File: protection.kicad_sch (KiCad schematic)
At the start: 29 parts, among them U21 LM339DR

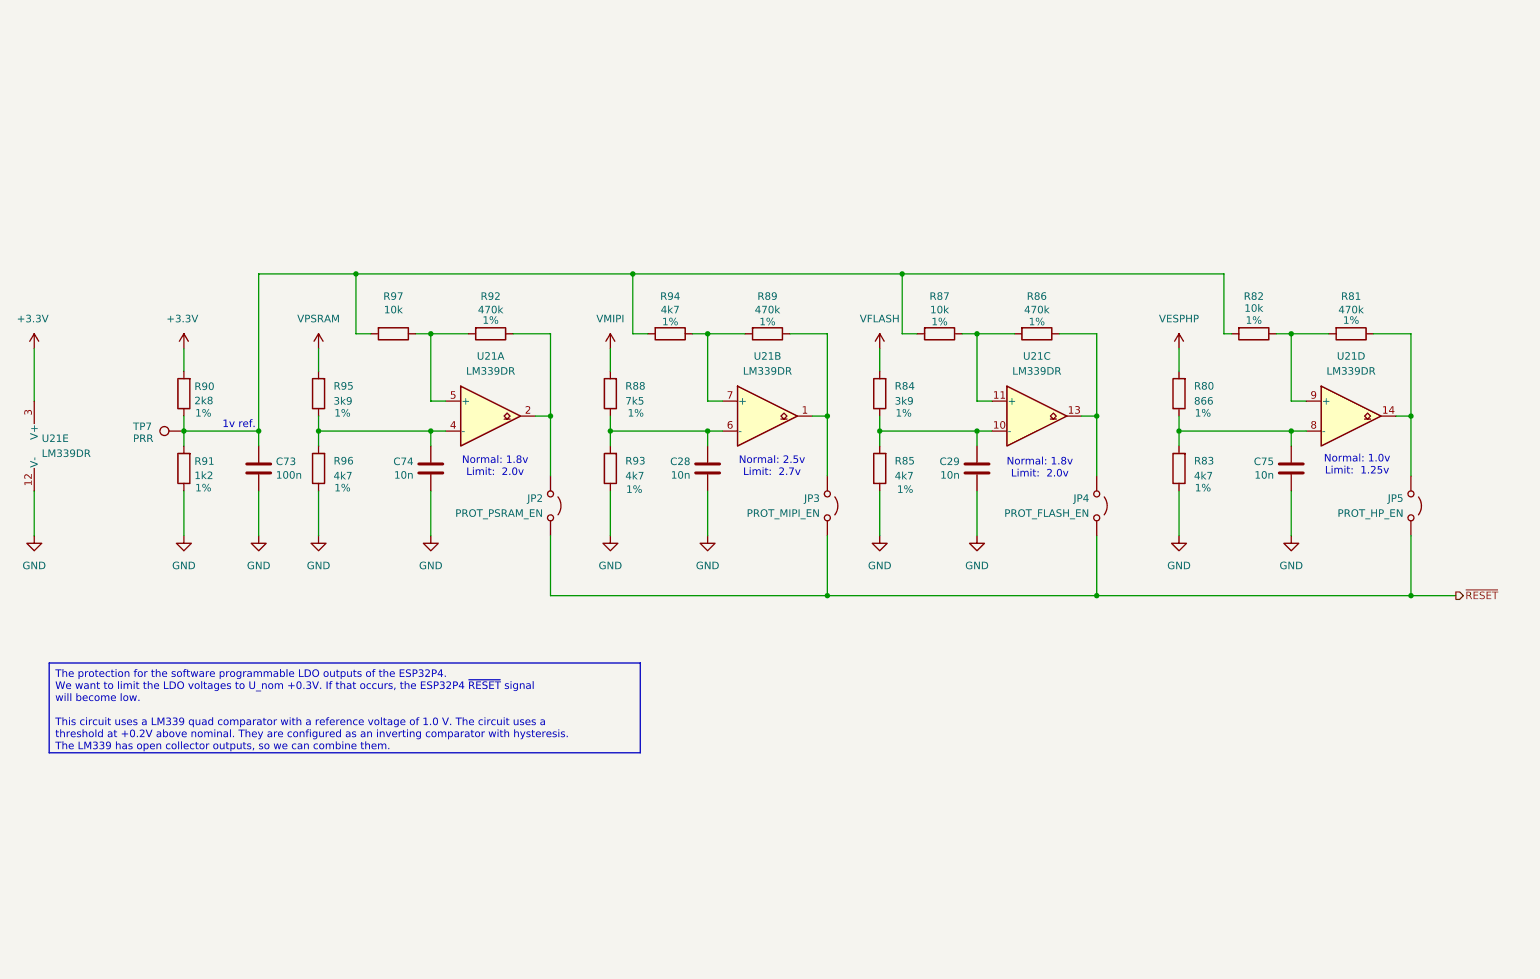
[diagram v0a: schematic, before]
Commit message: Replaced voltage comparitor circuit with zener setup. Also changed couple of 0.2mm vias to 0.3
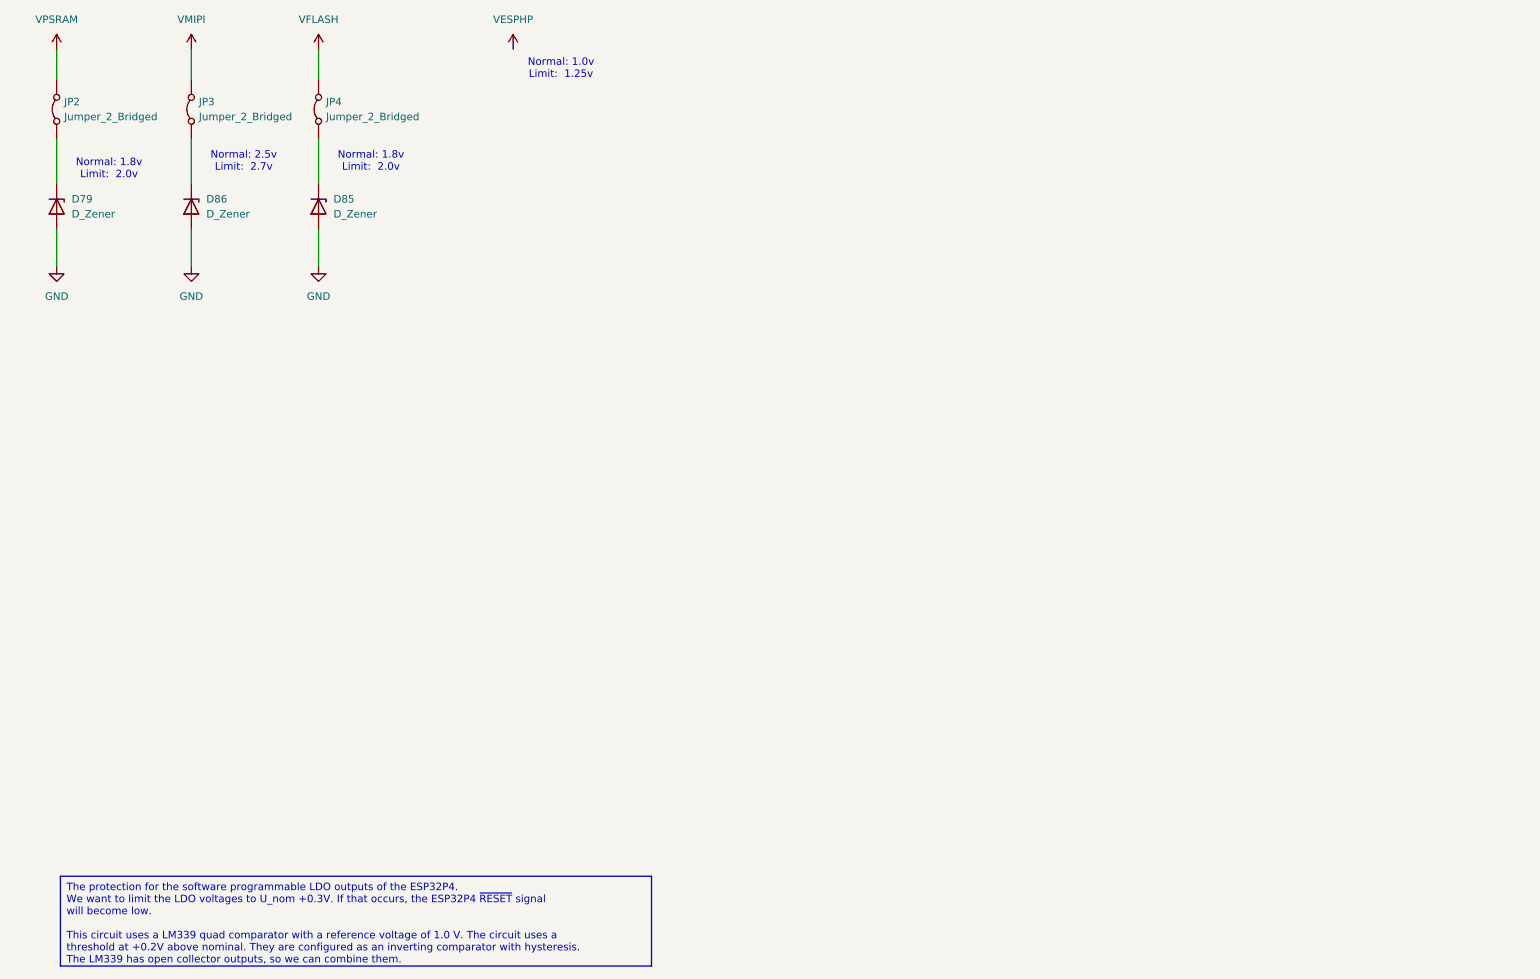
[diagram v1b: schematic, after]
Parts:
- removed C28, C29, C74, C75: 10n, Capacitor_SMD:C_0402_1005Metric, symbol symbols:C
- removed C73: 100n, Capacitor_SMD:C_0402_1005Metric, symbol symbols:C
- removed JP2: PROT_PSRAM_EN, Jumper:SolderJumper-2_P1.3mm_Open_RoundedPad1.0x1.5mm, symbol Jumper:Jumper_2_Open
- removed JP3: PROT_MIPI_EN, Jumper:SolderJumper-2_P1.3mm_Open_RoundedPad1.0x1.5mm, symbol Jumper:Jumper_2_Open
- removed JP4: PROT_FLASH_EN, Jumper:SolderJumper-2_P1.3mm_Open_RoundedPad1.0x1.5mm, symbol Jumper:Jumper_2_Open
- removed JP5: PROT_HP_EN, Jumper:SolderJumper-2_P1.3mm_Open_RoundedPad1.0x1.5mm, symbol Jumper:Jumper_2_Open
- removed R80: 866, Resistor_SMD:R_0402_1005Metric, symbol Device:R
- removed R81, R86, R89, R92: 470k, Resistor_SMD:R_0402_1005Metric, symbol Device:R
- removed R82, R87, R97: 10k, Resistor_SMD:R_0402_1005Metric, symbol Device:R
- removed R83, R85, R93, R94, R96: 4k7, Resistor_SMD:R_0402_1005Metric, symbol Device:R
- removed R84, R95: 3k9, Resistor_SMD:R_0402_1005Metric, symbol Device:R
- removed R88: 7k5, Resistor_SMD:R_0402_1005Metric, symbol Device:R
- removed R90: 2k8, Resistor_SMD:R_0402_1005Metric, symbol Device:R
- removed R91: 1k2, Resistor_SMD:R_0402_1005Metric, symbol Device:R
- removed TP7: PRR, TestPoint:TestPoint_Pad_D1.0mm, symbol Connector:TestPoint
- removed U21: LM339DR, Package_SO:SOIC-14_3.9x8.7mm_P1.27mm, symbol Comparator:LM339
- added D79, D85: D_Zener, Diode_SMD:D_SOD-123, symbol Device:D_Zener
- added D86: D_Zener, Diode_SMD:D_SOD-323F, symbol Device:D_Zener
- added JP2, JP3, JP4: Jumper_2_Bridged, Jumper:SolderJumper-2_P1.3mm_Bridged_RoundedPad1.0x1.5mm, symbol Jumper:Jumper_2_Bridged
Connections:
- net GND: now also D79.2 (A), D85.2 (A), D86.2 (A)
- net VFLASH: now also JP4.2 (B)
- net VMIPI: now also JP3.2 (B)
- net VPSRAM: now also JP2.2 (B)
- new net: D79.1 (K), JP2.1 (A)
- new net: D85.1 (K), JP4.1 (A)
- new net: D86.1 (K), JP3.1 (A)
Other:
- note removed: "1v ref."

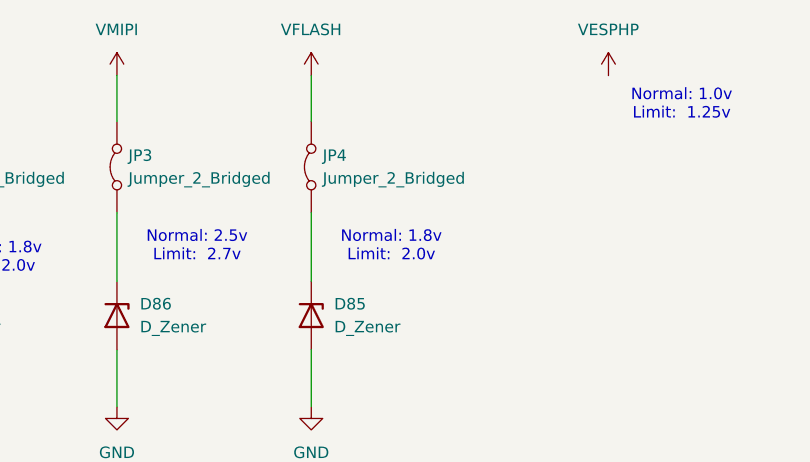
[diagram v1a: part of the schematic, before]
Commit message: Move protection diode for VFLASH, solve DRC errors, clean up
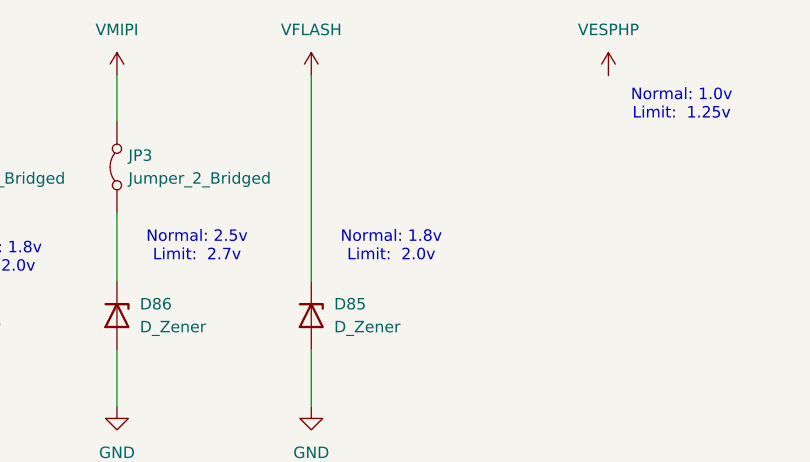
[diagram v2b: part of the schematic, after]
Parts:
- removed JP4: Jumper_2_Bridged, Jumper:SolderJumper-2_P1.3mm_Bridged_RoundedPad1.0x1.5mm, symbol Jumper:Jumper_2_Bridged
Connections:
- net VFLASH: now also D85.1 (K)
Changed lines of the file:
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@@
 	(wire
 		(pts
-			(xy 74.93 43.18) (xy 74.93 50.8)
+			(xy 74.93 27.94) (xy 74.93 50.8)
 		)
 		(stroke
@@
 		(pts
 			(xy 30.48 43.18) (xy 30.48 50.8)
-		)
-		(stroke
-			(width 0)
-			(type default)
-		)
-	)
-	(wire
-		(pts
-			(xy 74.93 27.94) (xy 74.93 33.02)
 		)
 		(stroke
@@
 					(unit 1)
 				)
-			)
-		)
-	)
-	(symbol
-		(lib_id "Jumper:Jumper_2_Bridged")
-		(at 74.93 38.1 90)
-		(unit 1)
-		(exclude_from_sim yes)
-		(in_bom yes)
-		(on_board yes)
-		(dnp no)
-		(fields_autoplaced yes)
-		(property "Reference" "JP4"
-			(at 76.2 36.8299 90)
-			(effects
-				(font
-					(size 1.27 1.27)
-				)
-				(justify right)
-			)
-		)
-		(property "Value" "Jumper_2_Bridged"
-			(at 76.2 39.3699 90)
-			(effects
-				(font
-					(size 1.27 1.27)
-				)
-				(justify right)
-			)
-		)
-		(property "Footprint" "Jumper:SolderJumper-2_P1.3mm_Bridged_RoundedPad1.0x1.5mm"
-			(at 74.93 38.1 0)
-			(effects
-				(font
-					(size 1.27 1.27)
-				)
-				(hide yes)
-			)
-		)
-		(property "Datasheet" "~"
-			(at 74.93 38.1 0)
-			(effects
-				(font
-					(size 1.27 1.27)
-				)
-				(hide yes)
-			)
-		)
-		(property "Description" "Jumper, 2-pole, closed/bridged"
-			(at 74.93 38.1 0)
-			(effects
-				(font
-					(size 1.27 1.27)
-				)
-				(hide yes)
-			)
-		)
-		(pin "1"
-		)
-		(pin "2"
-		)
-		(instances
-			(project "why2025"
-				(path "/6a31734e-65de-48f3-8156-2b24b665b183/3d60835a-4261-467a-b239-9fb76f6e13a1/ff07b197-d1d2-4b00-87d3-a97f534a0288"
-					(reference "JP4")
-					(unit 1)
-				)
